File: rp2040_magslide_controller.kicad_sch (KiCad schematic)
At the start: 1 part

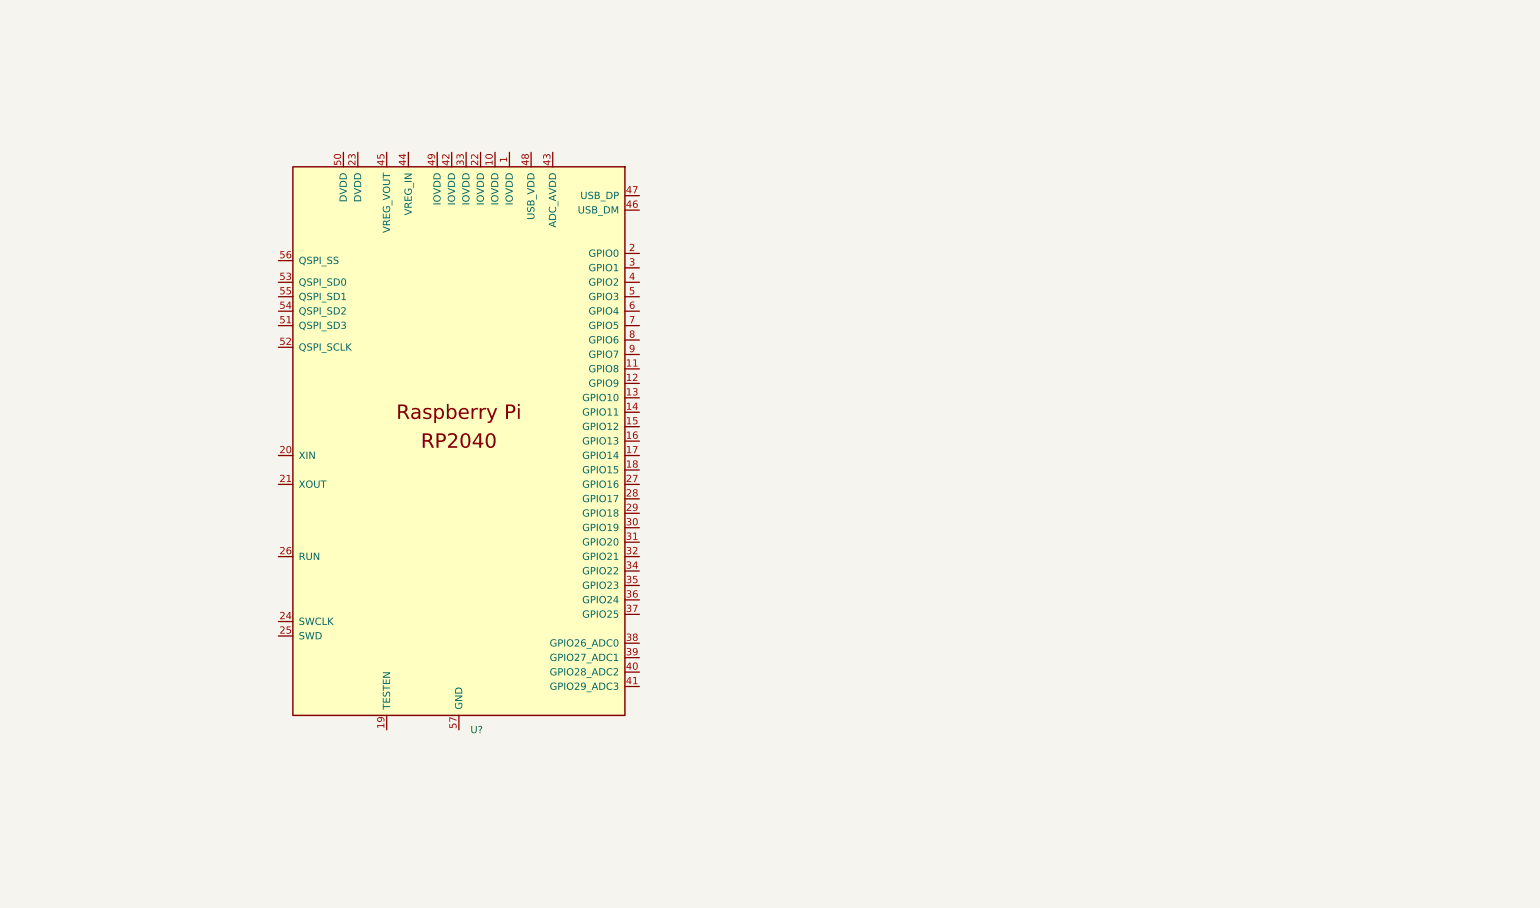
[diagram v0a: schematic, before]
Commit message: Inc
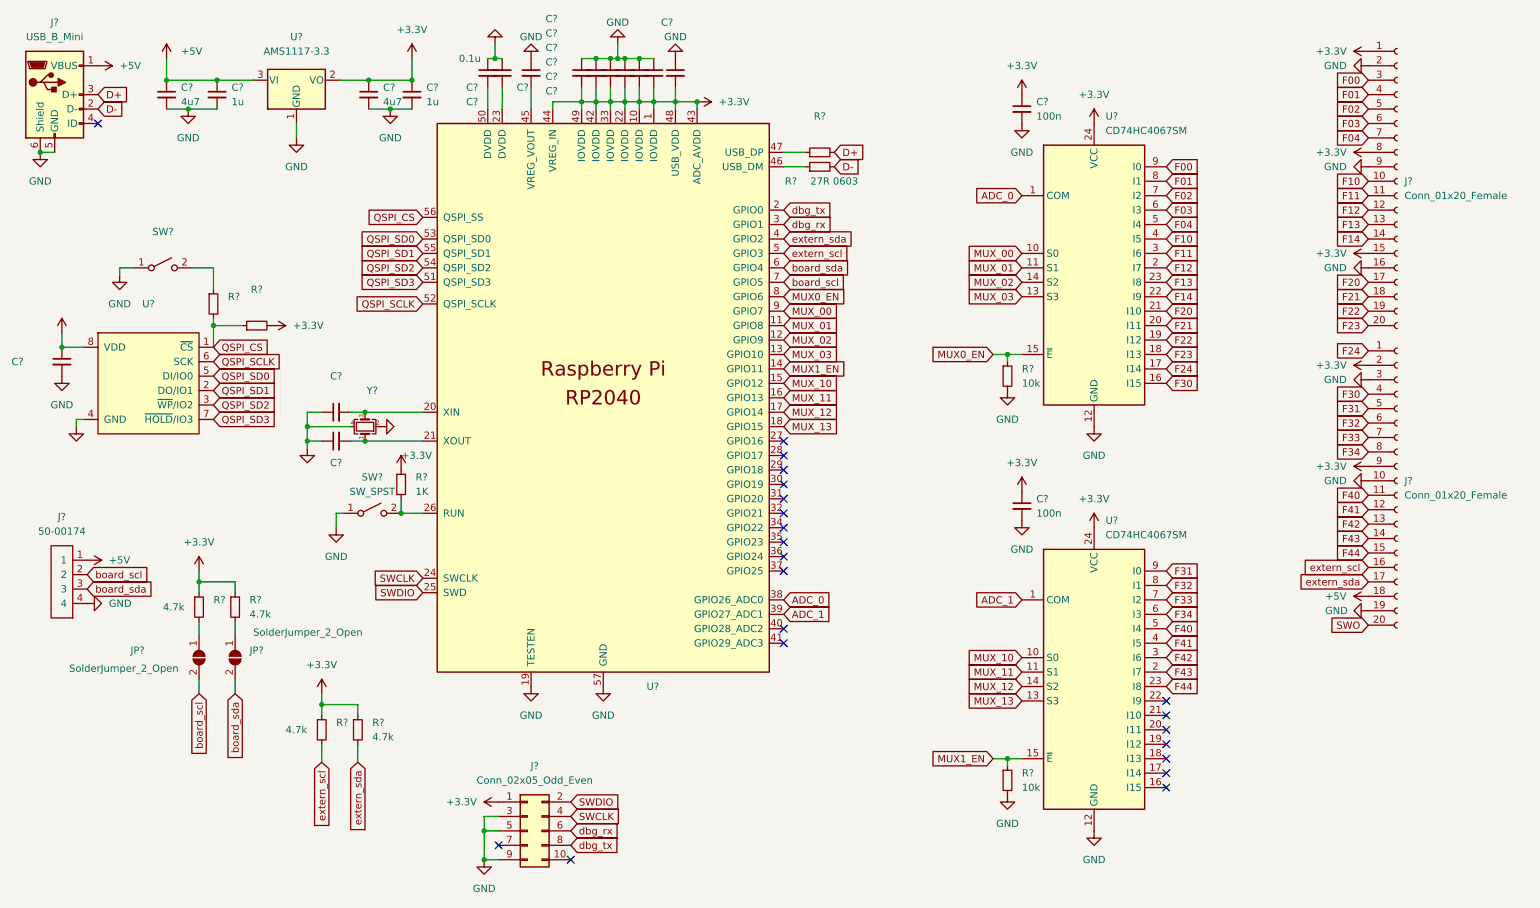
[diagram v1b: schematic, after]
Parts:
- added C? (x12): (no value), symbol Device:C_Small
- added C?: 0.1u, symbol Device:C_Small
- added C? (x2): 4u7, Capacitor_SMD:C_0603_1608Metric, symbol Device:C_Small
- added C? (x2): 1u, Capacitor_SMD:C_0603_1608Metric, symbol Device:C_Small
- added C? (x2): 100n, Capacitor_SMD:C_0402_1005Metric, symbol Device:C_Small
- added J? (x2): Conn_01x20_Female, misc:20_pin_header, symbol Connector:Conn_01x20_Female
- added J?: USB_B_Mini, Connector_USB:USB_Micro-B_Molex-105017-0001, symbol Connector:USB_B_Mini
- added J?: 50-00174, misc:54-00174, symbol misc:50-00174
- added J?: Conn_02x05_Odd_Even, Connector:Tag-Connect_TC2050-IDC-NL_2x05_P1.27mm_Vertical, symbol Connector_Generic:Conn_02x05_Odd_Even
- added JP? (x2): SolderJumper_2_Open, Jumper:SolderJumper-2_P1.3mm_Open_TrianglePad1.0x1.5mm, symbol Jumper:SolderJumper_2_Open
- added R? (x3): (no value), symbol Device:R_Small
- added R? (x2): 10k, Resistor_SMD:R_0402_1005Metric, symbol Device:R_Small
- added R? (x4): 4.7k, Resistor_SMD:R_0402_1005Metric, symbol Device:R_Small
- added R?: 27R 0603, symbol Device:R_Small
- added R?: 1K, symbol Device:R_Small
- added SW?: (no value), symbol Switch:SW_SPST
- added SW?: SW_SPST, symbol Switch:SW_SPST
- added U? (x2): CD74HC4067SM, Package_SO:SSOP-24_5.3x8.2mm_P0.65mm, symbol 74xx:CD74HC4067SM
- added U?: (no value), symbol Memory_Flash_Extra:W25Q64JV
- added U?: AMS1117-3.3, Package_TO_SOT_SMD:SOT-223-3_TabPin2, symbol Regulator_Linear:AMS1117-3.3
- added Y?: (no value), symbol Device:Crystal_GND24_Small
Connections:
- net +3V3: now reaches U?.1 (IOVDD)
- net +3V3: now also U?.10 (IOVDD), U?.22 (IOVDD), U?.33 (IOVDD), U?.42 (IOVDD), U?.43 (ADC_AVDD), U?.44 (VREG_IN), U?.48 (USB_VDD), U?.49 (IOVDD), C?.1, C?.1, C?.1, C?.1, C?.1, C?.2, C?.2, C?.2, C?.2, C?.2, C?.2, C?.2, J?.1 (Pin_1), J?.1 (Pin_1), J?.15 (Pin_15), J?.2 (Pin_2), J?.8 (Pin_8), J?.9 (Pin_9), R?.1, R?.1, R?.1, R?.1, R?.1, R?.2, U?.2 (VO), U?.24 (VCC), U?.24 (VCC), U?.8 (VDD)
- net MUX_01: now reaches U?.11 (GPIO8)
- net MUX_01: now also U?.11 (S1)
- net MUX_02: now reaches U?.12 (GPIO9)
- net MUX_02: now also U?.14 (S2)
- net MUX_03: now reaches U?.13 (GPIO10)
- net MUX_03: now also U?.13 (S3)
- net MUX1_EN: now reaches U?.14 (GPIO11)
- net MUX1_EN: now also R?.1, U?.15 (~{E})
- net MUX_10: now reaches U?.15 (GPIO12)
- net MUX_10: now also U?.10 (S0)
- net MUX_11: now reaches U?.16 (GPIO13)
- net MUX_11: now also U?.11 (S1)
- net MUX_12: now reaches U?.17 (GPIO14)
- net MUX_12: now also U?.14 (S2)
- net MUX_13: now reaches U?.18 (GPIO15)
- net MUX_13: now also U?.13 (S3)
- net GND: now reaches U?.19 (TESTEN)
- net GND: now also U?.57 (GND), C?.1, C?.1, C?.1, C?.1, C?.1, C?.1, C?.1, C?.1, C?.1, C?.1, C?.1, C?.1, C?.2, C?.2, C?.2, C?.2, C?.2, C?.2, C?.2, J?.10 (Pin_10), J?.16 (Pin_16), J?.19 (Pin_19), J?.2 (Pin_2), J?.3 (Pin_3), J?.3 (Pin_3), J?.4, J?.5 (GND), J?.5 (Pin_5), J?.6 (Shield), J?.9 (Pin_9), J?.9 (Pin_9), R?.2, R?.2, SW?.1 (A), SW?.1 (A), U?.1 (GND), U?.12 (GND), U?.12 (GND), U?.4 (GND), U?.9 (GND), Y?.2, Y?.4
- net dbg_tx: now reaches U?.2 (GPIO0)
- net dbg_tx: now also J?.8 (Pin_8)
- net at U?.20 (XIN): now also C?.2, Y?.3
- net at U?.21 (XOUT): now also C?.2, Y?.1
- net at U?.23 (DVDD): now also C?.2
- net SWCLK: now reaches U?.24 (SWCLK)
- net SWCLK: now also J?.4 (Pin_4)
- net SWDIO: now reaches U?.25 (SWD)
- net SWDIO: now also J?.2 (Pin_2)
- net at U?.26 (RUN): now also R?.2, SW?.2 (B)
- net dbg_rx: now reaches U?.3 (GPIO1)
- net dbg_rx: now also J?.6 (Pin_6)
- net ADC_0: now reaches U?.38 (GPIO26_ADC0)
- net ADC_0: now also U?.1 (COM)
- net ADC_1: now reaches U?.39 (GPIO27_ADC1)
- net ADC_1: now also U?.1 (COM)
- net extern_sda: now reaches U?.4 (GPIO2)
- net extern_sda: now also J?.17 (Pin_17), R?.2
- net at U?.45 (VREG_VOUT): now also C?.2
- net at U?.46 (USB_DM): now also R?.1
- net at U?.47 (USB_DP): now also R?.1
- net extern_scl: now reaches U?.5 (GPIO3)
- net extern_scl: now also J?.16 (Pin_16), R?.2
- net at U?.50 (DVDD): now also C?.2
- net QSPI_SD3: now reaches U?.51 (QSPI_SD3)
- net QSPI_SD3: now also U?.7 (~{HOLD}/IO3)
- net QSPI_SCLK: now reaches U?.52 (QSPI_SCLK)
- net QSPI_SCLK: now also U?.6 (SCK)
- net QSPI_SD0: now reaches U?.53 (QSPI_SD0)
- net QSPI_SD0: now also U?.5 (DI/IO0)
- net QSPI_SD2: now reaches U?.54 (QSPI_SD2)
- net QSPI_SD2: now also U?.3 (~{WP}/IO2)
- net QSPI_SD1: now reaches U?.55 (QSPI_SD1)
- net QSPI_SD1: now also U?.2 (DO/IO1)
- net QSPI_CS: now reaches U?.56 (QSPI_SS)
- net QSPI_CS: now also R?.1, R?.2, U?.1 (~{CS})
- net board_sda: now reaches U?.6 (GPIO4)
- net board_sda: now also J?.3, JP?.2 (B)
- net board_scl: now reaches U?.7 (GPIO5)
- net board_scl: now also J?.2, JP?.2 (B)
- net MUX0_EN: now reaches U?.8 (GPIO6)
- net MUX0_EN: now also R?.1, U?.15 (~{E})
- net MUX_00: now reaches U?.9 (GPIO7)
- net MUX_00: now also U?.10 (S0)
- new net: R?.1, SW?.2 (B)
- new net: JP?.1 (A), R?.2 (x2)
- new net +5V: C?.1, C?.1, J?.1, J?.1 (VBUS), J?.18 (Pin_18), U?.3 (VI)
- new net D+: J?.3 (D+), R?.2
- new net D-: J?.2 (D-), R?.2
- new net F00: J?.3 (Pin_3), U?.9 (I0)
- new net F01: J?.4 (Pin_4), U?.8 (I1)
- new net F02: J?.5 (Pin_5), U?.7 (I2)
- new net F03: J?.6 (Pin_6), U?.6 (I3)
- new net F04: J?.7 (Pin_7), U?.5 (I4)
- new net F10: J?.10 (Pin_10), U?.4 (I5)
- new net F11: J?.11 (Pin_11), U?.3 (I6)
- new net F12: J?.12 (Pin_12), U?.2 (I7)
- new net F13: J?.13 (Pin_13), U?.23 (I8)
- new net F14: J?.14 (Pin_14), U?.22 (I9)
- new net F20: J?.17 (Pin_17), U?.21 (I10)
- new net F21: J?.18 (Pin_18), U?.20 (I11)
- new net F22: J?.19 (Pin_19), U?.19 (I12)
- new net F23: J?.20 (Pin_20), U?.18 (I13)
- new net F24: J?.1 (Pin_1), U?.17 (I14)
- new net F30: J?.4 (Pin_4), U?.16 (I15)
- new net F31: J?.5 (Pin_5), U?.9 (I0)
- new net F32: J?.6 (Pin_6), U?.8 (I1)
- new net F33: J?.7 (Pin_7), U?.7 (I2)
- new net F34: J?.8 (Pin_8), U?.6 (I3)
- new net F40: J?.11 (Pin_11), U?.5 (I4)
- new net F41: J?.12 (Pin_12), U?.4 (I5)
- new net F42: J?.13 (Pin_13), U?.3 (I6)
- new net F43: J?.14 (Pin_14), U?.2 (I7)
- new net F44: J?.15 (Pin_15), U?.23 (I8)
- new net SWO: J?.20 (Pin_20)
- no-connect marks 0 -> 22
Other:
- moved on the sheet: U?
